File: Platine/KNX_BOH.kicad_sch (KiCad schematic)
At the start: 3 parts, among them U2 ESP32-DEVKITC-32D

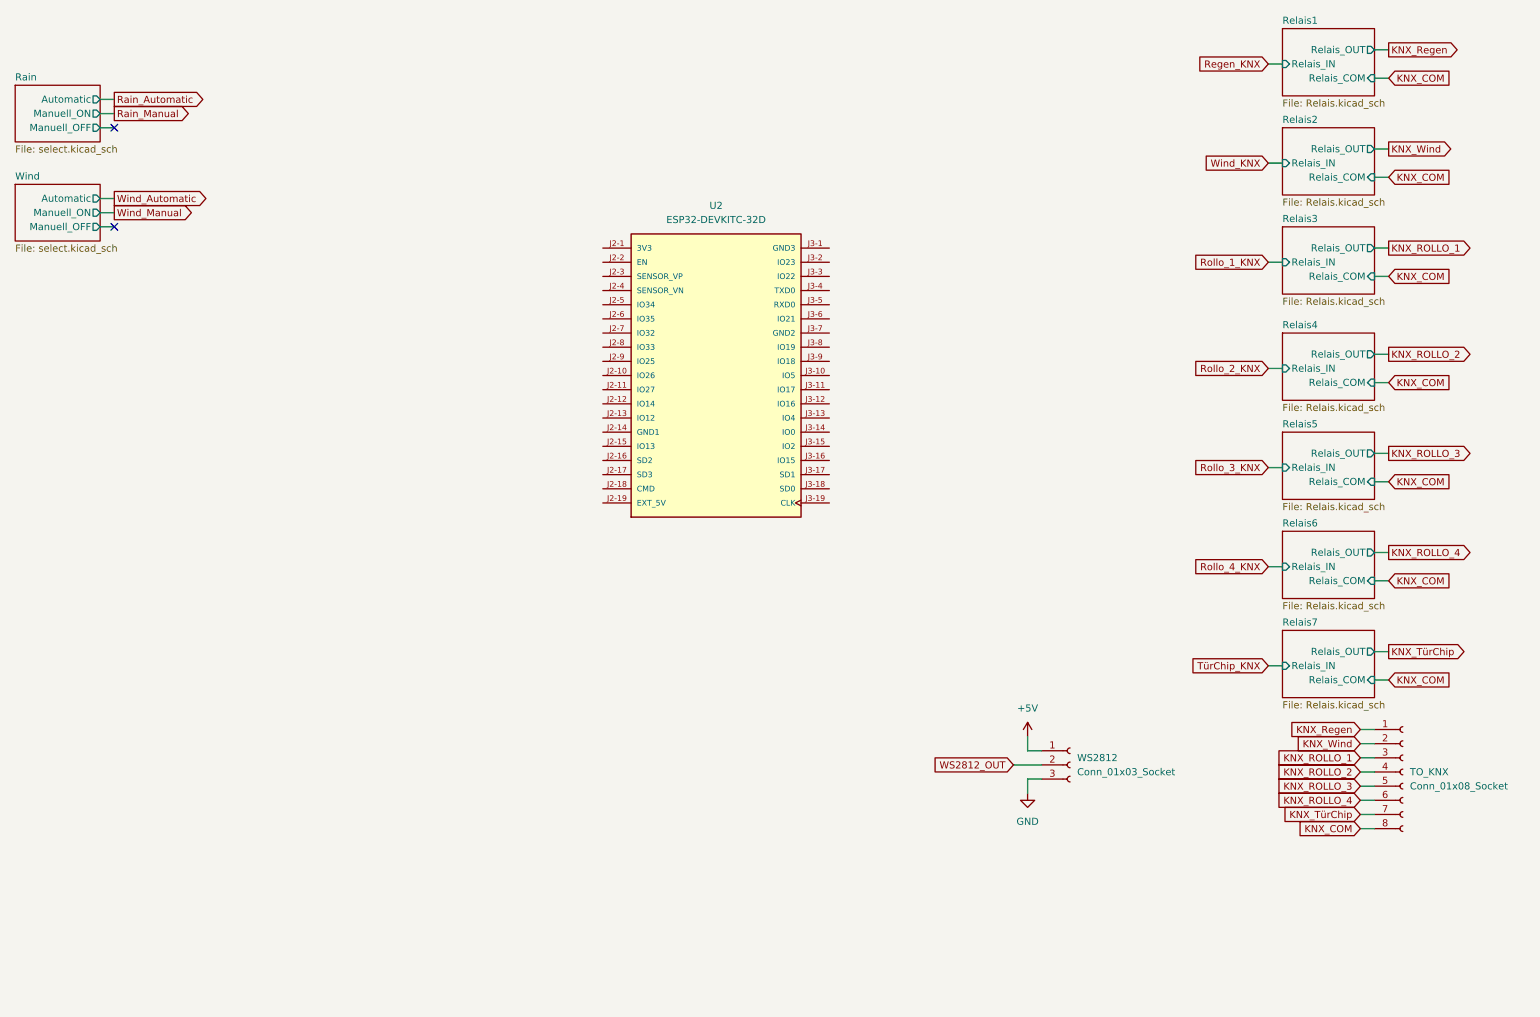
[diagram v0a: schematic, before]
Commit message: Platine fast fertig
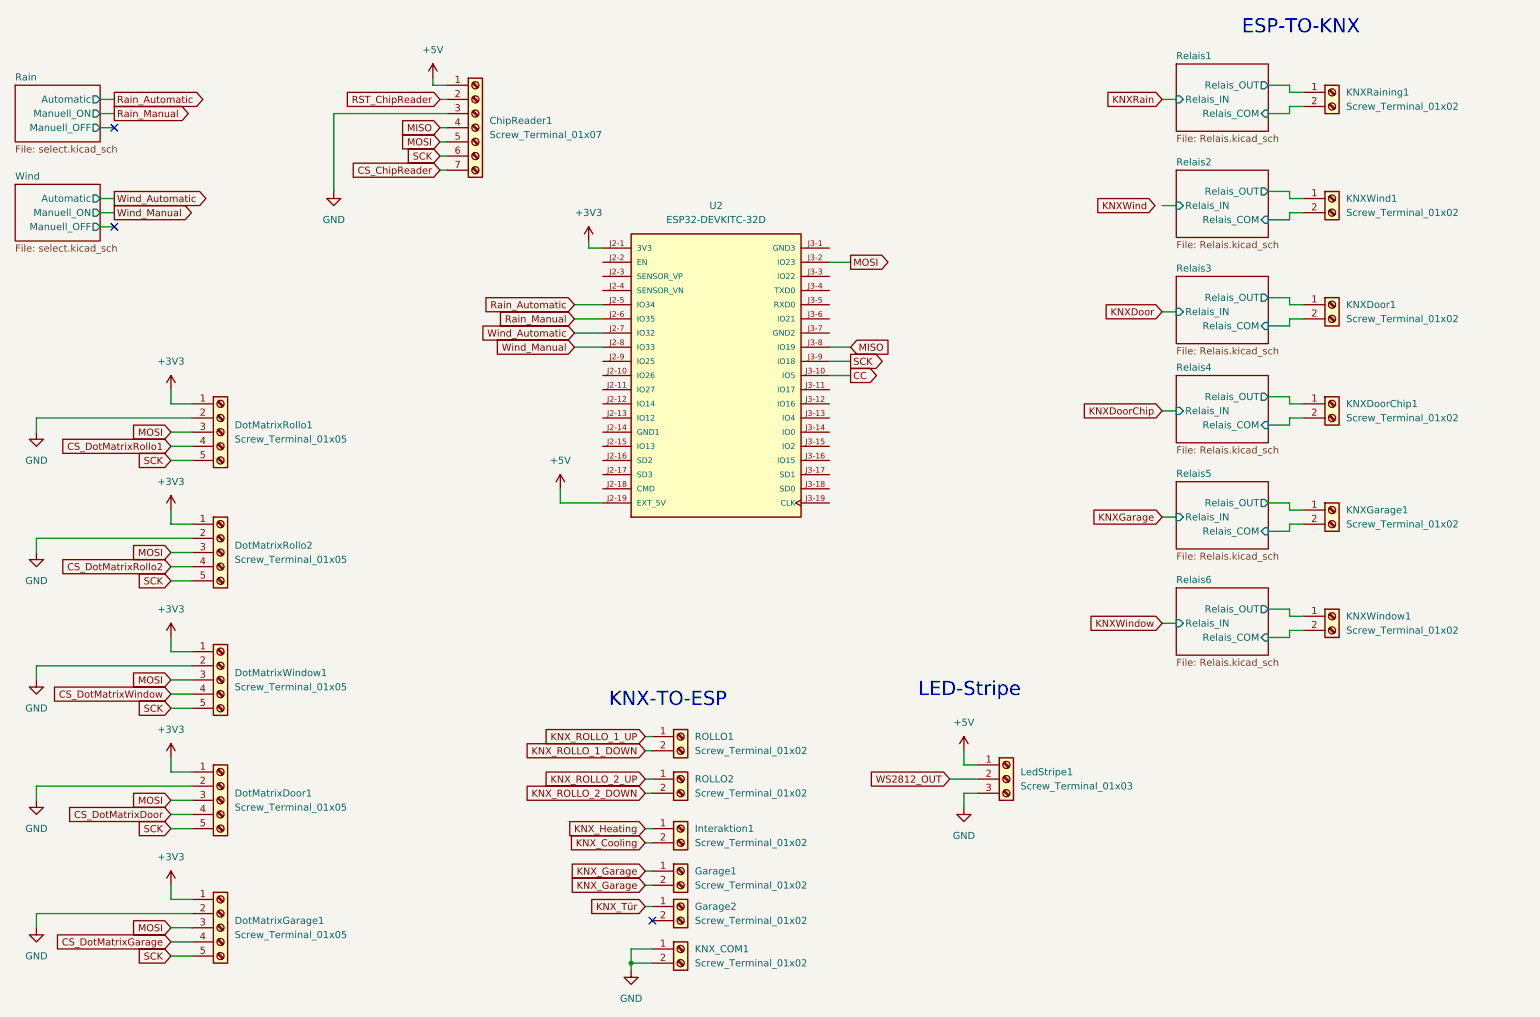
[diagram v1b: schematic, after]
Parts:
- removed TO_KNX: Conn_01x08_Socket, symbol Connector:Conn_01x08_Socket
- removed WS2812: Conn_01x03_Socket, symbol Connector:Conn_01x03_Socket
- added ChipReader1: Screw_Terminal_01x07, TerminalBlock_Phoenix:TerminalBlock_Phoenix_MKDS-1,5-7-5.08_1x07_P5.08mm_Horizontal, symbol Connector:Screw_Terminal_01x07
- added DotMatrixDoor1, DotMatrixGarage1, DotMatrixRollo1, DotMatrixRollo2, DotMatrixWindow1: Screw_Terminal_01x05, TerminalBlock_Phoenix:TerminalBlock_Phoenix_MPT-0,5-7-2.54_1x07_P2.54mm_Horizontal, symbol Connector:Screw_Terminal_01x05
- added Garage1, Garage2, Interaktion1, KNXDoor1, KNXDoorChip1, KNXGarage1, KNXRaining1, KNXWind1, KNXWindow1, KNX_COM1, ROLLO1, ROLLO2: Screw_Terminal_01x02, TerminalBlock_Phoenix:TerminalBlock_Phoenix_MKDS-1,5-2-5.08_1x02_P5.08mm_Horizontal, symbol Connector:Screw_Terminal_01x02
- added LedStripe1: Screw_Terminal_01x03, TerminalBlock_Phoenix:TerminalBlock_Phoenix_MKDS-1,5-3-5.08_1x03_P5.08mm_Horizontal, symbol Connector:Screw_Terminal_01x03
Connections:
- net +5V: now also U2.J2-19 (EXT_5V), ChipReader1.1 (Pin_1), LedStripe1.1 (Pin_1)
- net GND: now also ChipReader1.3 (Pin_3), DotMatrixDoor1.2 (Pin_2), DotMatrixGarage1.2 (Pin_2), DotMatrixRollo1.2 (Pin_2), DotMatrixRollo2.2 (Pin_2), DotMatrixWindow1.2 (Pin_2), KNX_COM1.1 (Pin_1), KNX_COM1.2 (Pin_2), LedStripe1.3 (Pin_3)
- net Rain_Automatic: now also U2.J2-5 (IO34)
- net Rain_Manual: now also U2.J2-6 (IO35)
- net WS2812_OUT: now also LedStripe1.2 (Pin_2)
- net Wind_Automatic: now also U2.J2-7 (IO32)
- net Wind_Manual: now also U2.J2-8 (IO33)
- net +3V3: now reaches U2.J2-1 (3V3)
- net +3V3: now also DotMatrixDoor1.1 (Pin_1), DotMatrixGarage1.1 (Pin_1), DotMatrixRollo1.1 (Pin_1), DotMatrixRollo2.1 (Pin_1), DotMatrixWindow1.1 (Pin_1)
- net CC: now reaches U2.J3-10 (IO5)
- net MOSI: now reaches U2.J3-2 (IO23)
- net MOSI: now also ChipReader1.5 (Pin_5), DotMatrixDoor1.3 (Pin_3), DotMatrixGarage1.3 (Pin_3), DotMatrixRollo1.3 (Pin_3), DotMatrixRollo2.3 (Pin_3), DotMatrixWindow1.3 (Pin_3)
- net MISO: now reaches U2.J3-8 (IO19)
- net MISO: now also ChipReader1.4 (Pin_4)
- net SCK: now reaches U2.J3-9 (IO18)
- net SCK: now also ChipReader1.6 (Pin_6), DotMatrixDoor1.5 (Pin_5), DotMatrixGarage1.5 (Pin_5), DotMatrixRollo1.5 (Pin_5), DotMatrixRollo2.5 (Pin_5), DotMatrixWindow1.5 (Pin_5)
- new net CS_ChipReader: ChipReader1.7 (Pin_7)
- new net CS_DotMatrixDoor: DotMatrixDoor1.4 (Pin_4)
- new net CS_DotMatrixGarage: DotMatrixGarage1.4 (Pin_4)
- new net CS_DotMatrixRollo1: DotMatrixRollo1.4 (Pin_4)
- new net CS_DotMatrixRollo2: DotMatrixRollo2.4 (Pin_4)
- new net CS_DotMatrixWindow: DotMatrixWindow1.4 (Pin_4)
- new net KNX_Cooling: Interaktion1.2 (Pin_2)
- new net KNX_Garage: Garage1.1 (Pin_1), Garage1.2 (Pin_2)
- new net KNX_Heating: Interaktion1.1 (Pin_1)
- new net KNX_ROLLO_1_DOWN: ROLLO1.2 (Pin_2)
- new net KNX_ROLLO_1_UP: ROLLO1.1 (Pin_1)
- new net KNX_ROLLO_2_DOWN: ROLLO2.2 (Pin_2)
- new net KNX_ROLLO_2_UP: ROLLO2.1 (Pin_1)
- new net KNX_Tür: Garage2.1 (Pin_1)
- new net RST_ChipReader: ChipReader1.2 (Pin_2)
- new net Relais1/Relais_COM: KNXRaining1.2 (Pin_2)
- new net Relais1/Relais_OUT: KNXRaining1.1 (Pin_1)
- new net Relais2/Relais_COM: KNXWind1.2 (Pin_2)
- new net Relais2/Relais_OUT: KNXWind1.1 (Pin_1)
- new net Relais3/Relais_COM: KNXDoor1.2 (Pin_2)
- new net Relais3/Relais_OUT: KNXDoor1.1 (Pin_1)
- new net Relais4/Relais_COM: KNXDoorChip1.2 (Pin_2)
- new net Relais4/Relais_OUT: KNXDoorChip1.1 (Pin_1)
- new net Relais5/Relais_COM: KNXGarage1.2 (Pin_2)
- new net Relais5/Relais_OUT: KNXGarage1.1 (Pin_1)
- new net Relais6/Relais_COM: KNXWindow1.2 (Pin_2)
- new net Relais6/Relais_OUT: KNXWindow1.1 (Pin_1)
- no-connect marks 2 -> 3
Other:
- removed sheet Relais7
- note added: "ESP-TO-KNX"
- note added: "KNX-TO-ESP"
- note added: "LED-Stripe"
